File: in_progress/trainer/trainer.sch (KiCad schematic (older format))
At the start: 54 parts, among them CON1 BARREL_JACK, P2 CONN_01X02, P3 CONN_01X03, P4 USB_A, P5 CONN_01X02, P6 CONN_01X03, P7 CONN_02X08, Q1 2N3904, U2 LM7805, U3 ULN2803A, U4 ULN2803A, X1 Buzzer_Son

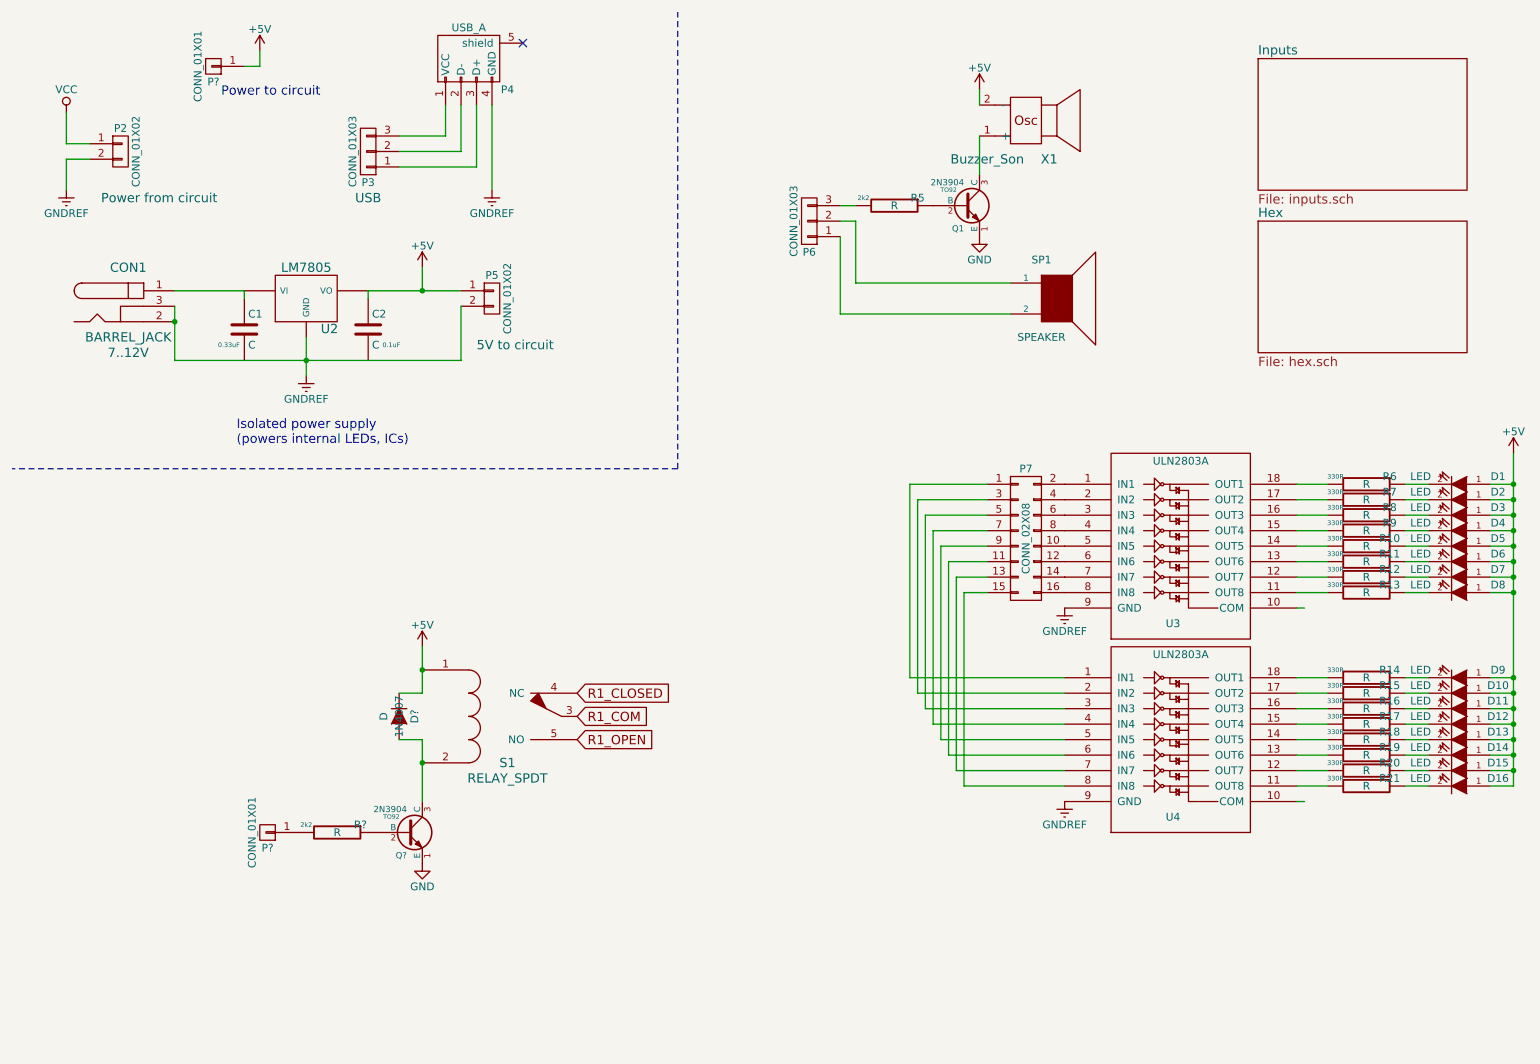
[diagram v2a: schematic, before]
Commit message: .
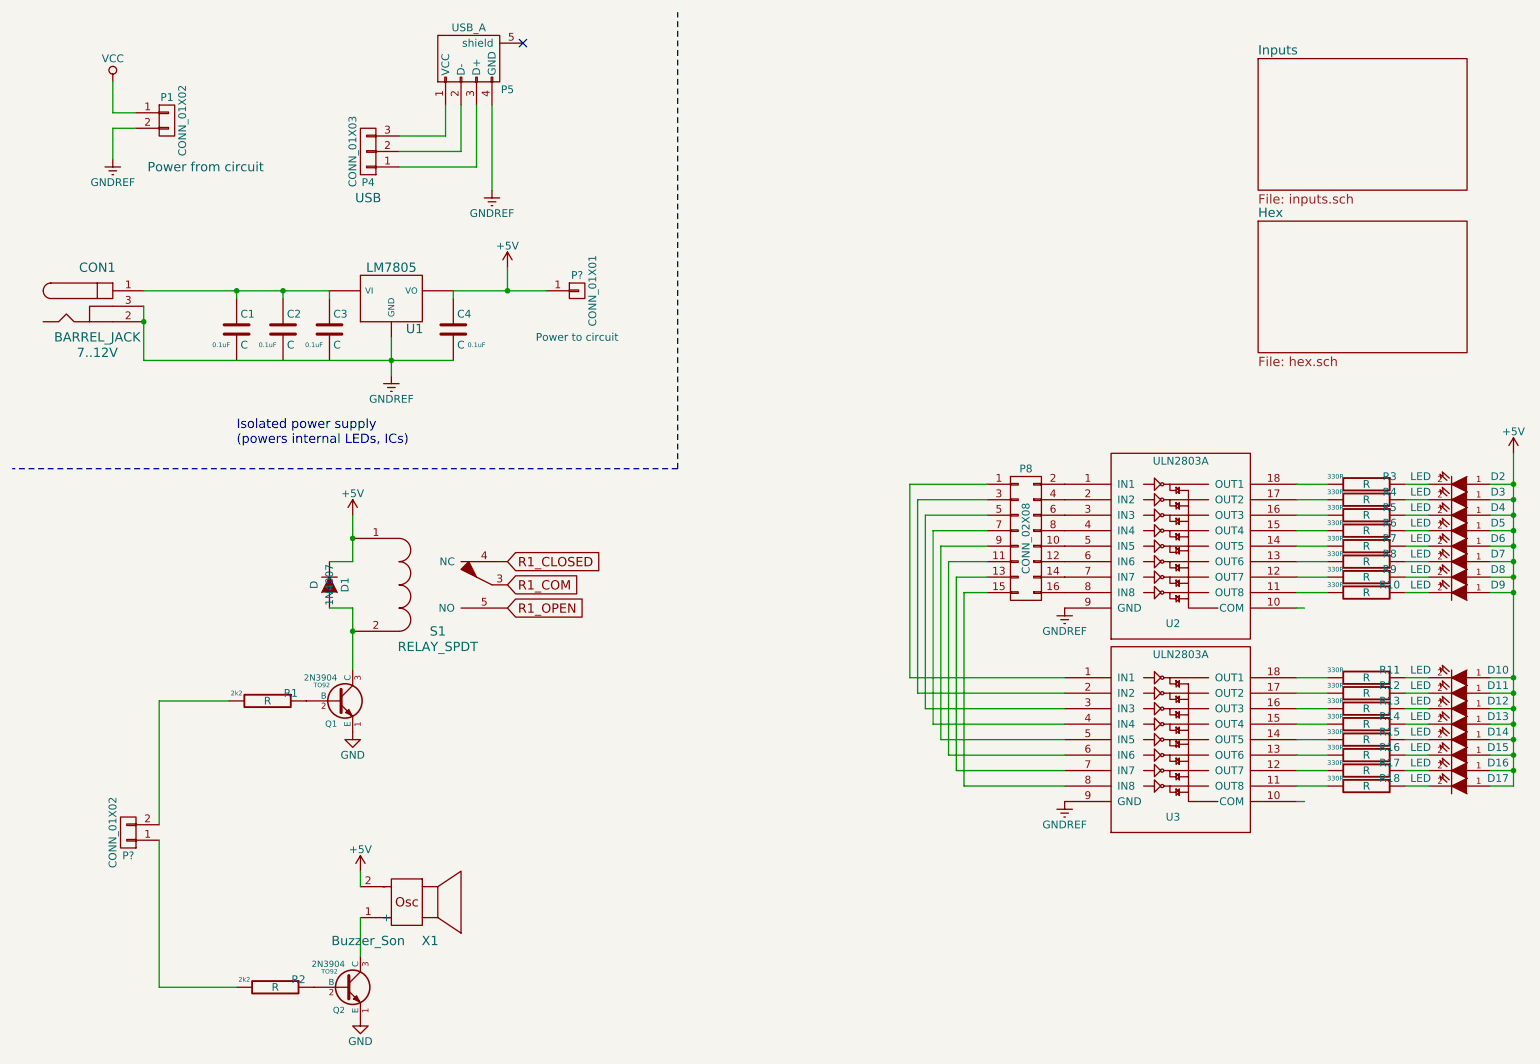
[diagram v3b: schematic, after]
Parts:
- removed P5: CONN_01X02, 5V to circuit, symbol CONN_01X02
- removed P6: CONN_01X03, symbol CONN_01X03
- removed P? (x2): CONN_01X01, symbol CONN_01X01
- removed SP1: SPEAKER, symbol SPEAKER
- added C1, C2: C, 0.1uF, symbol C-RESCUE-trainer
- added P?: CONN_01X01, Power to circuit, symbol CONN_01X01
- added P?: CONN_01X02, symbol CONN_01X02
- C3: renamed from C1; footprint 0.33uF -> 0.1uF
- gave numbers to parts that had none: 3
- renumbered C2 to C4, D9 to D10, D10 to D11, D11 to D12, D12 to D13, D13 to D14, D14 to D15, D15 to D16, D16 to D17, D1 to D2, D2 to D3, D3 to D4, D4 to D5, D5 to D6, D6 to D7, D7 to D8, D8 to D9, P2 to P1, P3 to P4, P4 to P5, P7 to P8, Q1 to Q2, R13 to R10, R14 to R11, R15 to R12, R16 to R13, R17 to R14, R18 to R15, R19 to R16, R20 to R17, R21 to R18, R5 to R2, R6 to R3, R7 to R4, R8 to R5, R9 to R6, R10 to R7, R11 to R8, R12 to R9, U2 to U1, U3 to U2, U4 to U3
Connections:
- net +5V: now also P?.1 (P1)
- net GNDREF: now also C4.2
- net at C3.1, CON1.1, U1.VI: now also C1.1, C2.1
- net at R2.2: now also P?.1 (P1)
- net at R1.2: now also P?.2 (P2)
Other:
- note removed: "Power to circuit"
- moved on the sheet: C3, C4, CON1, D1, P1, Q1, Q2, R1, R2, S1, U1, X1
